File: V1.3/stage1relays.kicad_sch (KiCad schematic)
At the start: 14 parts, among them T3 AO3400A, T4 AO3400A

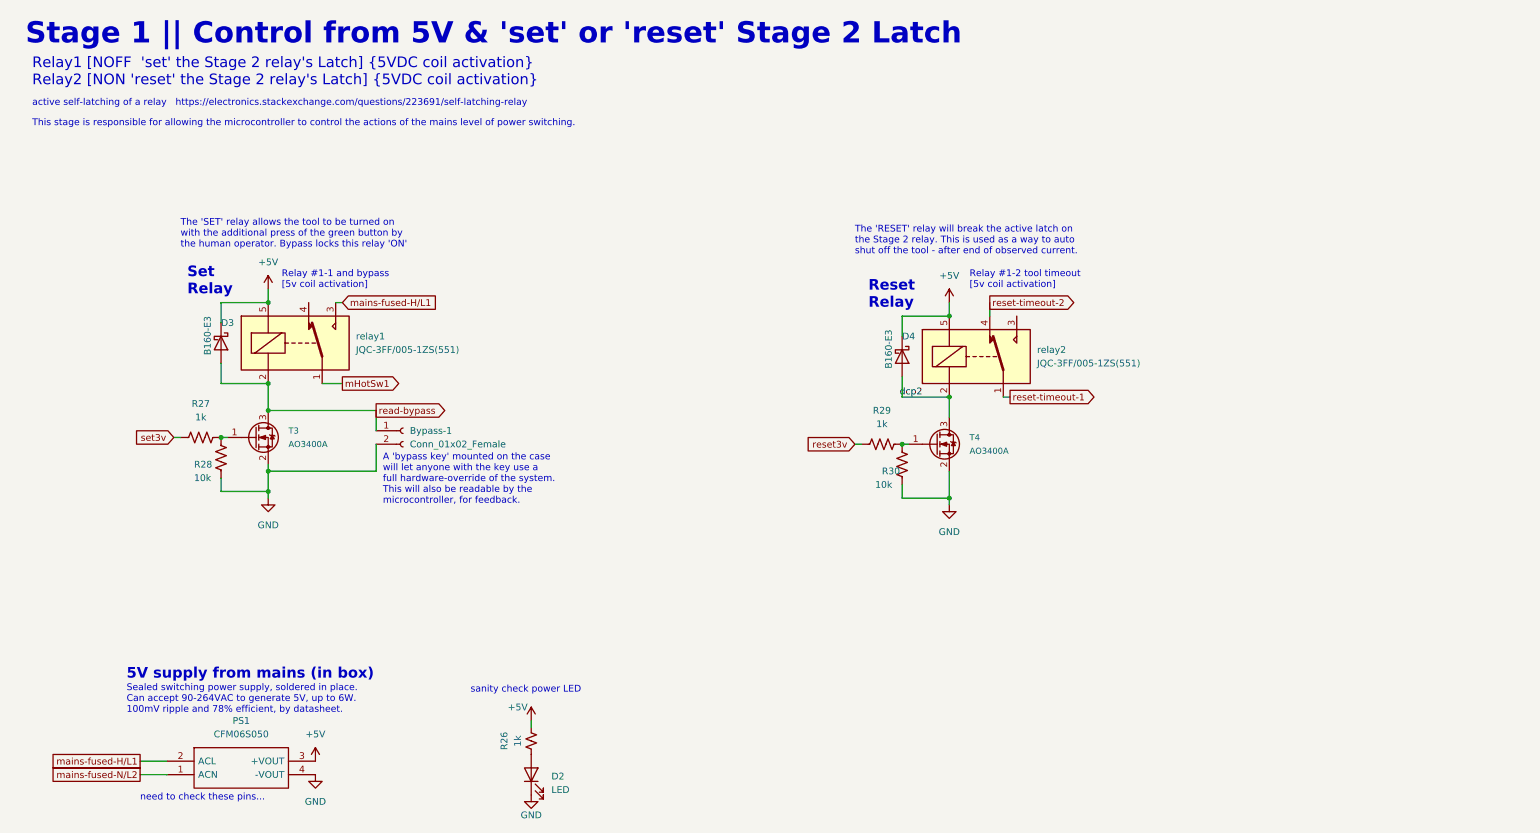
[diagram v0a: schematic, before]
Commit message: update v1.3 schematic documentation
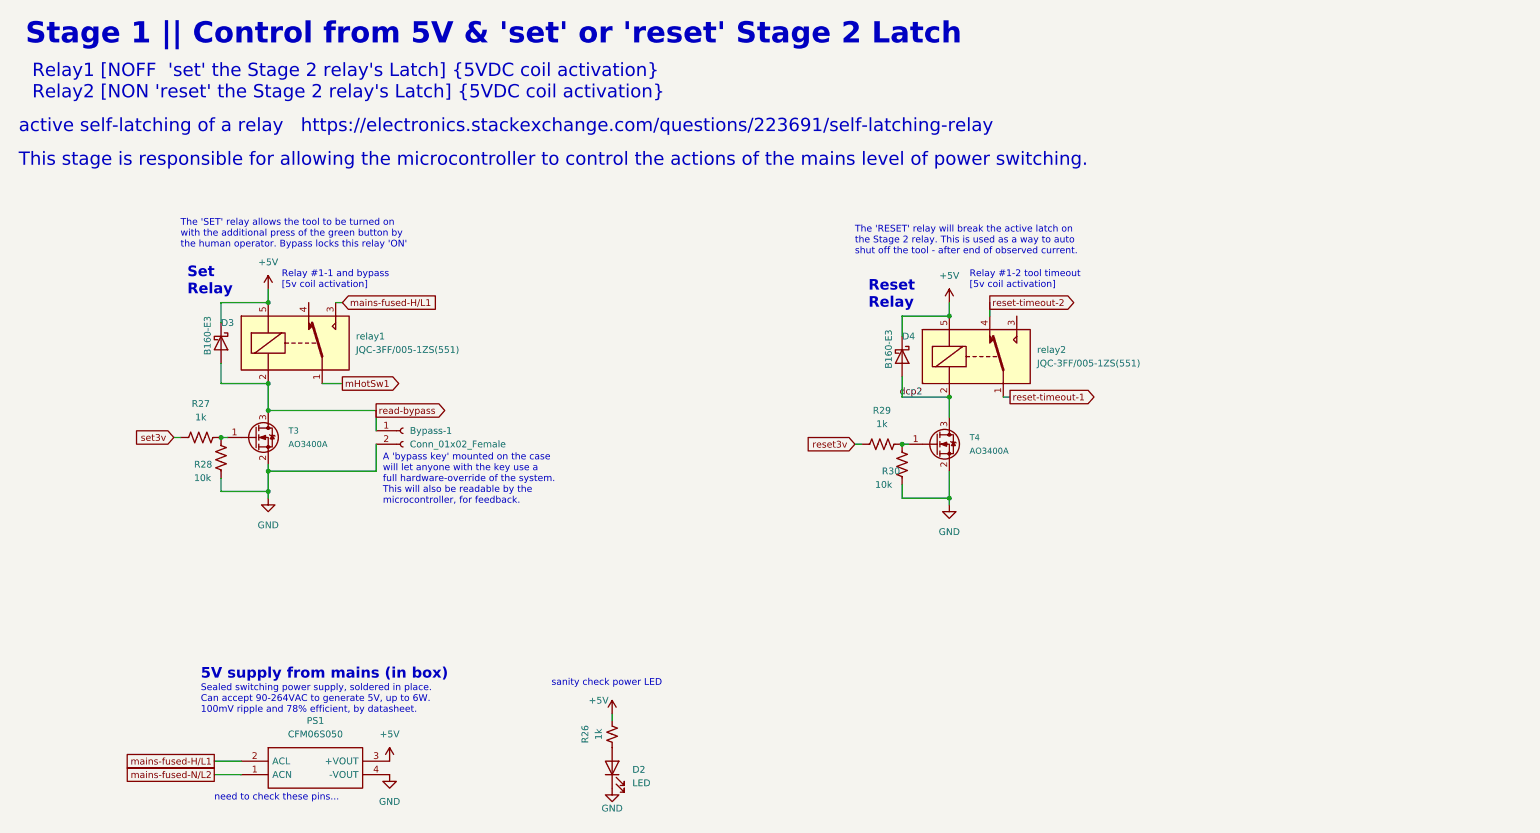
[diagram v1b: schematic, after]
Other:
- moved on the sheet: D2, PS1, R26
